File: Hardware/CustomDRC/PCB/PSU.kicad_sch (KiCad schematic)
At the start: 13 parts, among them U201 AP63203WU-7

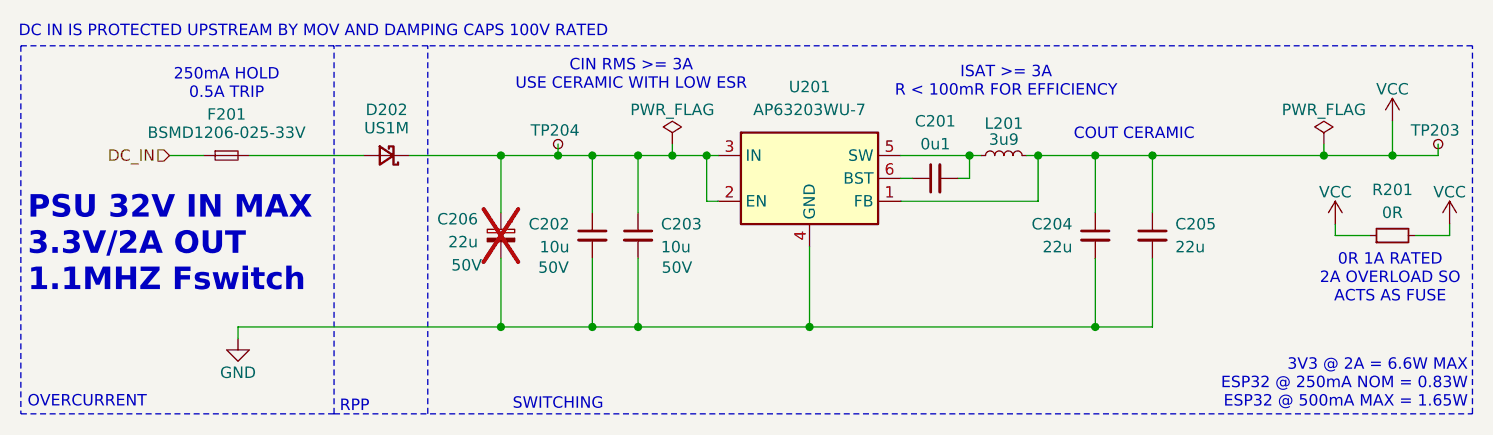
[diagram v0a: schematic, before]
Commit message: Update HW folder with latest work on rev B
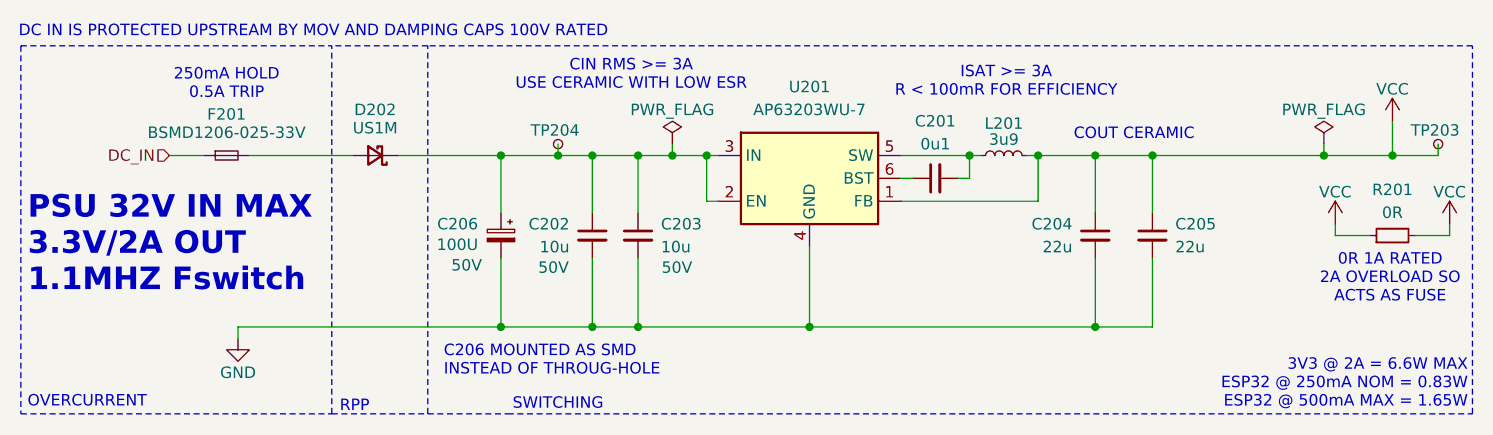
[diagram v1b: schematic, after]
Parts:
- C206: value 22u -> 100U; footprint Capacitor_SMD:CP_Elec_6.3x5.4_Nichicon -> CDRC_Footprints:Capacitor_D6.3xL12mm_SMD; LCSC (none) -> C160200; MPN (none) -> ERZ1HM101E12OT; Manufacturer (none) -> AISHI(Aihua Group); now fitted; now in the parts list
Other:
- note added: "C206 MOUNTED AS SMD INSTEAD OF THROUG-HOLE"
- moved on the sheet: D202
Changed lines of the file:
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@@
 	(title_block
 		(title "CDRC - Custom DRC for Bit 10D")
-		(date "01-11-2024")
+		(date "25-11-2024")
 		(rev "B")
 		(company "JS HW")
@@
 	(polyline
 		(pts
-			(xy 69.85 70.358) (xy 104.648 70.358)
+			(xy 69.85 70.358) (xy 104.394 70.358)
 		)
 		(stroke
@@
 	(polyline
 		(pts
-			(xy 69.85 111.252) (xy 104.648 111.252)
+			(xy 69.85 111.252) (xy 104.394 111.252)
 		)
 		(stroke
@@
 	(polyline
 		(pts
-			(xy 104.648 111.252) (xy 104.648 70.358)
+			(xy 104.394 111.252) (xy 104.394 70.358)
 		)
 		(stroke
@@
 	(polyline
 		(pts
-			(xy 104.648 111.252) (xy 123.952 111.252)
+			(xy 104.394 111.252) (xy 123.952 111.252)
 		)
 		(stroke
@@
 	(wire
 		(pts
-			(xy 113.03 82.55) (xy 123.19 82.55)
+			(xy 111.76 82.55) (xy 123.19 82.55)
 		)
 		(stroke
@@
 	(wire
 		(pts
-			(xy 95.25 82.55) (xy 107.95 82.55)
+			(xy 95.25 82.55) (xy 106.68 82.55)
 		)
 		(stroke
@@
 	(polyline
 		(pts
-			(xy 115.062 70.358) (xy 104.648 70.358)
+			(xy 115.062 70.358) (xy 104.394 70.358)
 		)
 		(stroke
@@
 				(color 255 0 255 1)
 			)
+		)
+	)
+	(text "C206 MOUNTED AS SMD \nINSTEAD OF THROUG-HOLE"
+		(exclude_from_sim no)
+		(at 116.84 105.41 0)
+		(effects
+			(font
+				(size 1.27 1.27)
+				(color 255 0 255 1)
+			)
+			(justify left)
 		)
 	)
@@
 	(symbol
 		(lib_id "Device:D_Schottky_Small")
-		(at 110.49 82.55 180)
+		(at 109.22 82.55 180)
 		(unit 1)
 		(exclude_from_sim no)
@@
 		(dnp no)
 		(property "Reference" "D202"
-			(at 110.49 77.47 0)
+			(at 109.22 77.47 0)
 			(effects
 				(font
@@
 		)
 		(property "Value" "US1M"
-			(at 110.49 79.502 0)
+			(at 109.22 79.502 0)
 			(effects
 				(font
@@
 		)
 		(property "Footprint" "Diode_SMD:D_SMA_Handsoldering"
-			(at 110.49 82.55 90)
+			(at 109.22 82.55 90)
 			(effects
 				(font
@@
 		)
 		(property "Datasheet" "~"
-			(at 110.49 82.55 90)
+			(at 109.22 82.55 90)
 			(effects
 				(font
@@
 		)
 		(property "Description" "Schottky diode, small symbol"
-			(at 110.49 82.55 0)
+			(at 109.22 82.55 0)
 			(effects
 				(font
@@
 		)
 		(property "LCSC" "C412437"
-			(at 110.49 82.55 0)
+			(at 109.22 82.55 0)
 			(effects
 				(font
@@
 		)
 		(property "MPN" "US1M"
-			(at 110.49 82.55 0)
+			(at 109.22 82.55 0)
 			(effects
 				(font
@@
 		)
 		(property "Manufacturer" "MDD(Microdiode Semiconductor)"
-			(at 110.49 82.55 0)
+			(at 109.22 82.55 0)
 			(effects
 				(font
@@
 		(unit 1)
 		(exclude_from_sim no)
-		(in_bom no)
+		(in_bom yes)
 		(on_board yes)
-		(dnp yes)
+		(dnp no)
 		(property "Reference" "C206"
-			(at 120.65 89.6239 0)
+			(at 120.65 90.17 0)
 			(effects
 				(font
@@
 			)
 		)
-		(property "Value" "22u"
-			(at 120.65 92.1639 0)
+		(property "Value" "100U"
+			(at 120.65 92.456 0)
 			(effects
 				(font
@@
 			)
 		)
-		(property "Footprint" "Capacitor_SMD:CP_Elec_6.3x5.4_Nichicon"
+		(property "Footprint" "CDRC_Footprints:Capacitor_D6.3xL12mm_SMD"
 			(at 123.19 91.44 0)
 			(effects
@@
 			)
 		)
+		(property "MPN" "ERZ1HM101E12OT"
+			(at 123.19 91.44 0)
+			(effects
+				(font
+					(size 1.27 1.27)
+				)
+				(hide yes)
+			)
+		)
+		(property "Manufacturer" "AISHI(Aihua Group)"
+			(at 123.19 91.44 0)
+			(effects
+				(font
+					(size 1.27 1.27)
+				)
+				(hide yes)
+			)
+		)
+		(property "LCSC" "C160200"
+			(at 123.19 91.44 0)
+			(effects
+				(font
+					(size 1.27 1.27)
+				)
+				(hide yes)
+			)
+		)
